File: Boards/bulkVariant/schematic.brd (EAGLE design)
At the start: 93 x 70 mm, 99 parts, among them IC1 LM2596S, J1 AVR_SPI_PRG_6NS, U1 MAGJACK-POE, U2 MAGJACK-POE

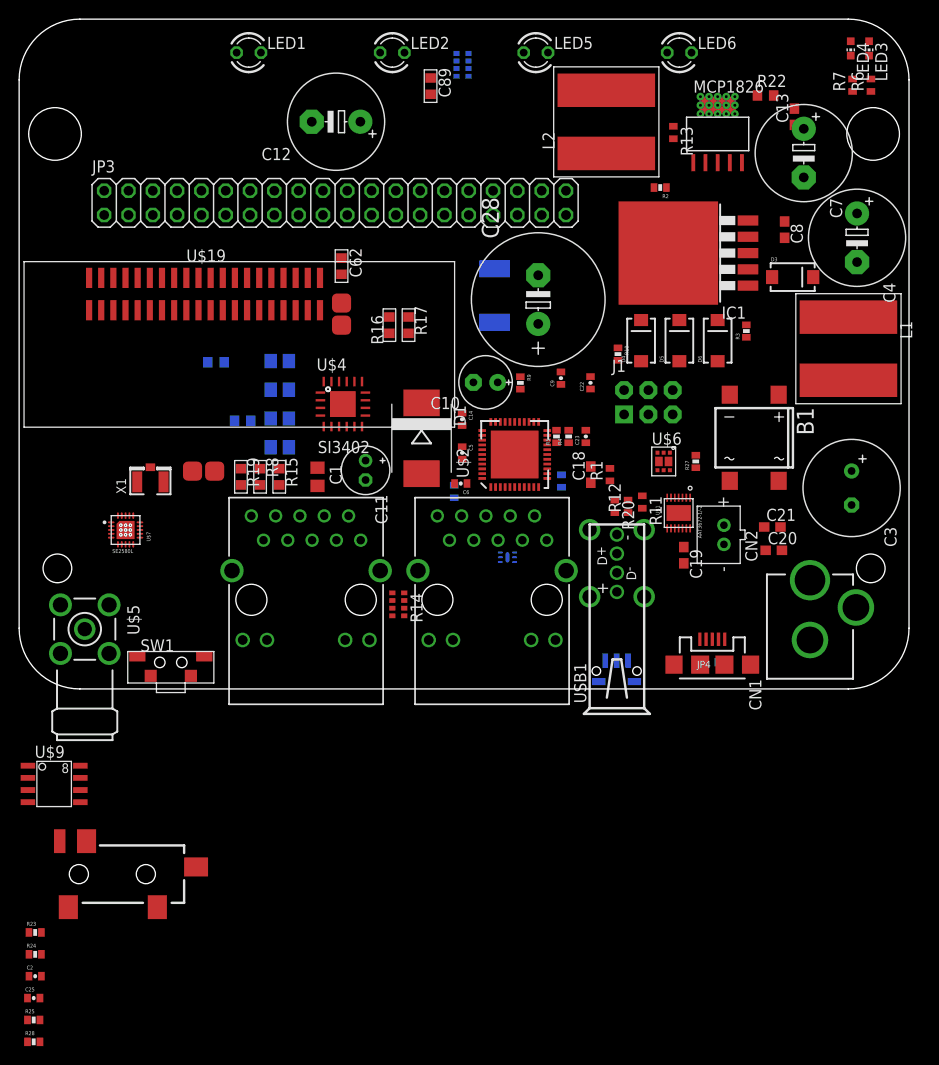
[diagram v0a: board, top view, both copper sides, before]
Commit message: normal Push.
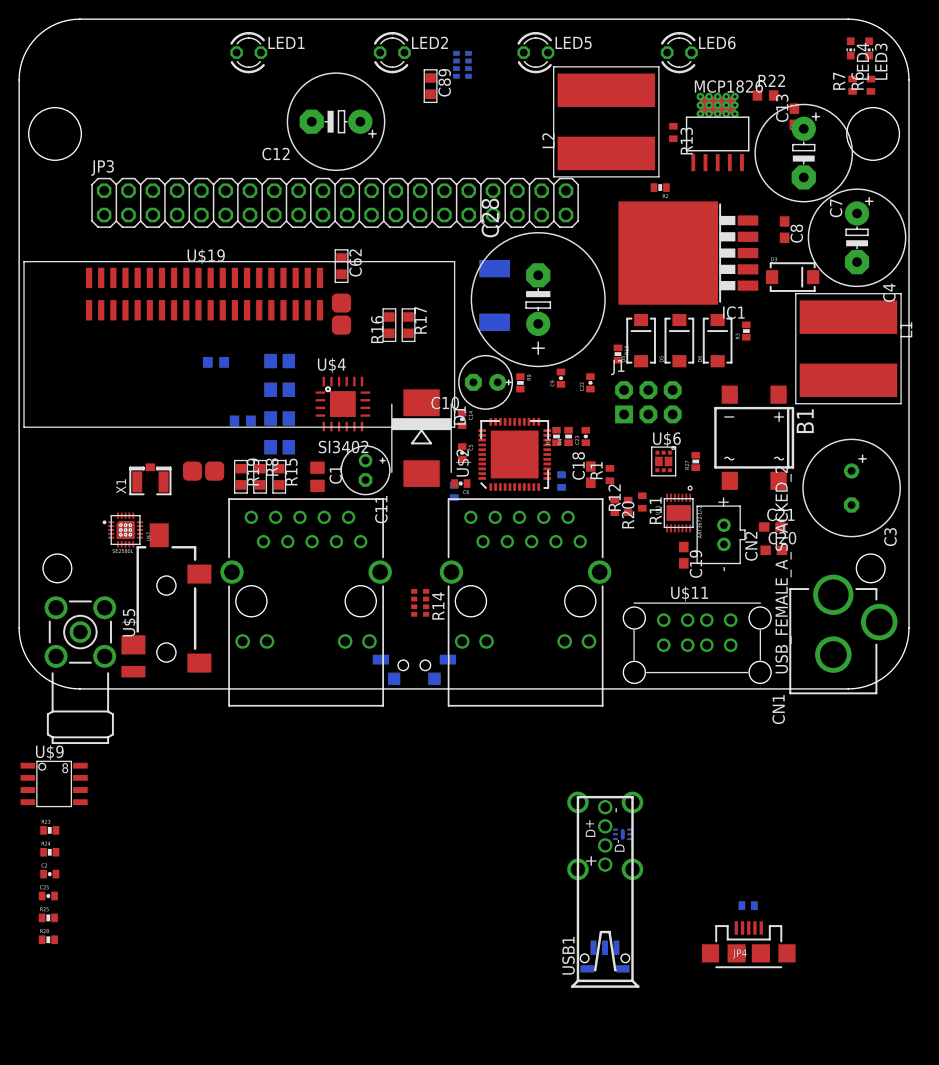
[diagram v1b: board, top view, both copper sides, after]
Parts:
- added U$11: USB_FEMALE_A_STACKED_2, schematic:USB_A_FEMALE_STACKED_2
- moved U$3 31.4 mm to (63.1, -15.2)
- moved JP4 30.4 mm to (76.3, -27.6)
- moved V- 30.0 mm to (61.2, -29.3)
- moved USB1 28.5 mm to (57.8, -31.1)
- moved C29 25.7 mm to (76.2, -22.7)
- moved SW1 25.5 mm to (41.3, 1.07), flipped to the bottom
- moved JP1 23.4 mm to (15.4, 0.30), turned to 90 degrees
- moved R23 10.8 mm to (3.20, -14.8)
- moved C2 10.8 mm to (3.20, -19.4)
- moved C25 10.8 mm to (3.05, -21.6)
- moved R24 10.8 mm to (3.20, -17.1)
- moved R25 10.8 mm to (3.05, -23.9)
- moved R28 10.8 mm to (3.05, -26.2)
- moved U1 3.51 mm to (52.9, 9.04)
- moved CN1 2.88 mm to (85.1, -3.76)
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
